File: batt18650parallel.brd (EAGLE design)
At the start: 89.8 x 62.2 mm, 6 parts

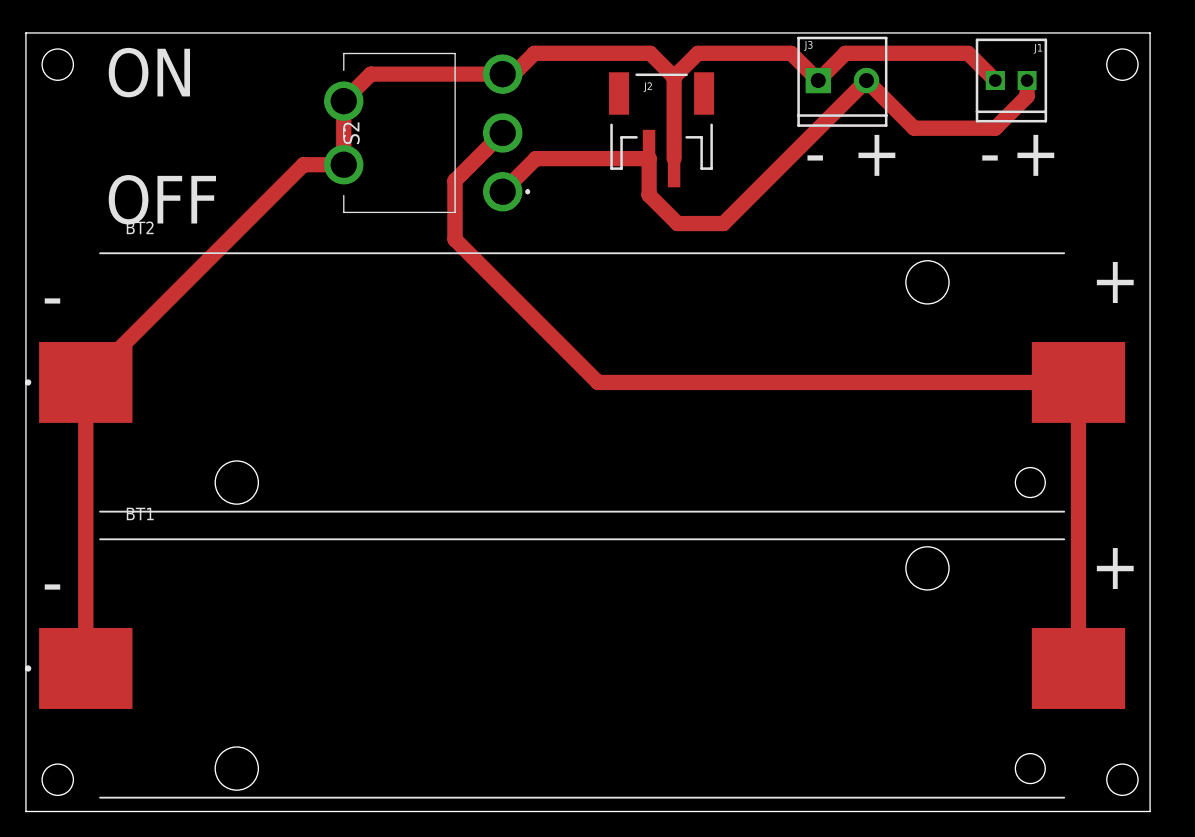
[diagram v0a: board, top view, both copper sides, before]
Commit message: Bobby Schulz design review: address
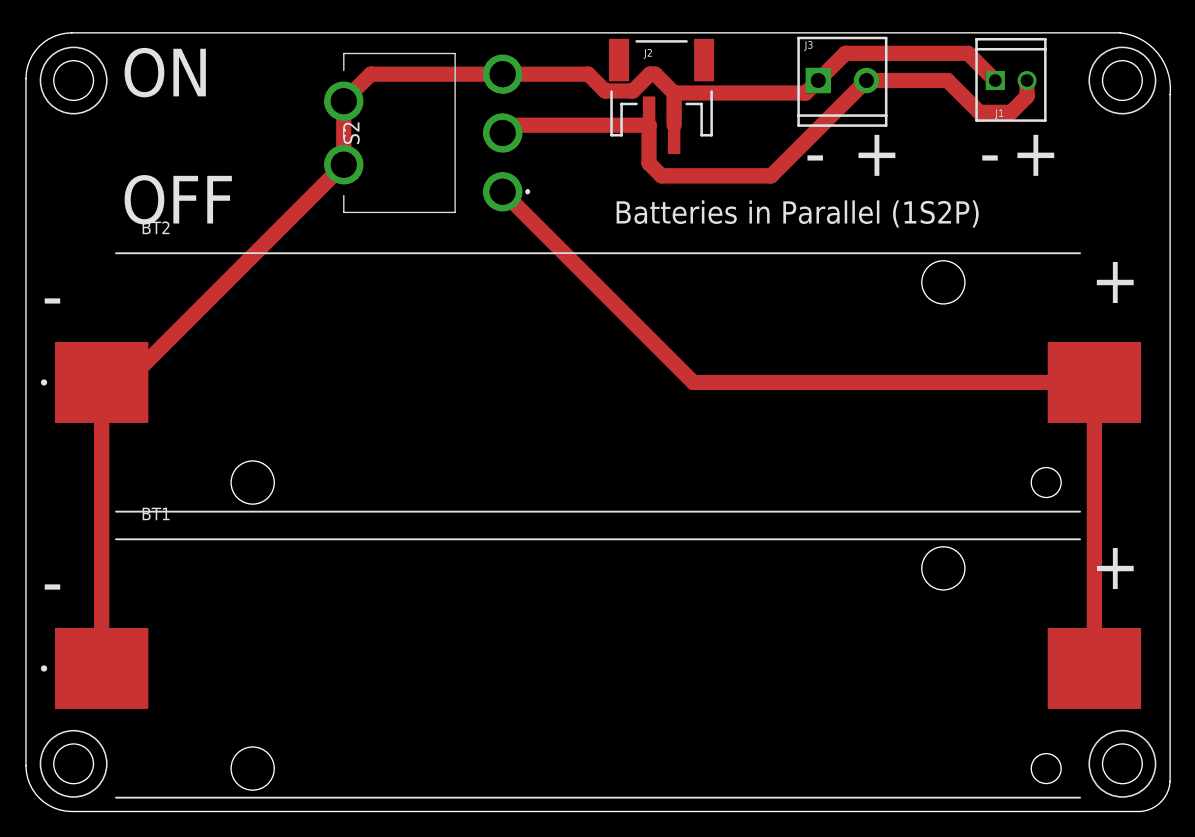
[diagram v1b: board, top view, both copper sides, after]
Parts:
- added H1, H2, H3, H4: (no value), bschulz:4_40
- J1: device SparkFun-Connectors:1X02_2.54_SCREWTERM -> bschulz:1X02_2.54_SCREWTERM
- moved J2 2.67 mm to (50.8, 58.5)
- moved J1 1.27 mm to (78.7, 58.4), turned to 0 degrees
- moved BT1 1.27 mm to (45.7, 11.4)
- moved BT2 1.27 mm to (45.7, 34.3)
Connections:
- net B+: now also S2.1; no longer S2.2
- net GND: now also J1.P2; no longer J1.P1
- net VCC: now also J1.P1, S2.2; no longer J1.P2, S2.1
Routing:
- net B+: track 87.5 -> 76.5 mm
- net GND: track 120.6 -> 115.0 mm
- net VCC: track 55.5 -> 51.6 mm
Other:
- board size 89.8 x 62.2 mm -> 91.5 x 62.2 mm
- board text added: "Batteries in Parallel (1S2P)"
